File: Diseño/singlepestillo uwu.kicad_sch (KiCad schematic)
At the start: 17 parts, among them J1 MAX98357A, J2 Conn_01x03_Pin, J3 Screw_Terminal_01x03, J5 Screw_Terminal_01x02, J9 Screw_Terminal_01x03, K3 G6AU, Q6 MMBT2222A, U3 EL817, U5 L7805, U6 ESP32DevKitv1

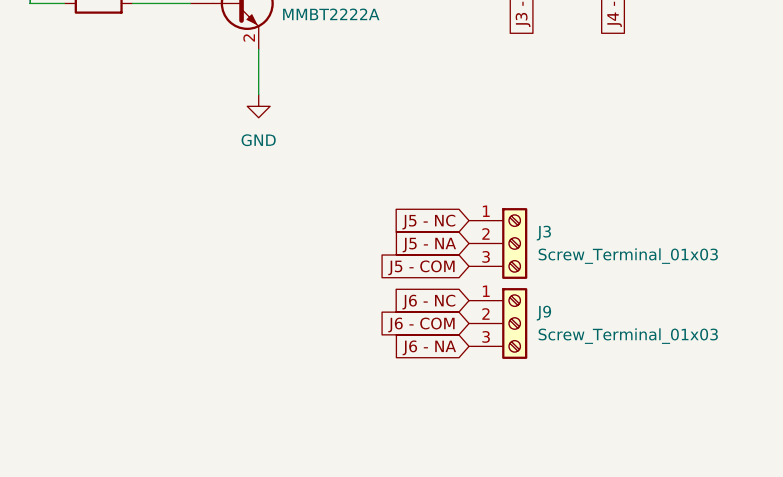
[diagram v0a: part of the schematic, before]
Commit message: avance pcb armado
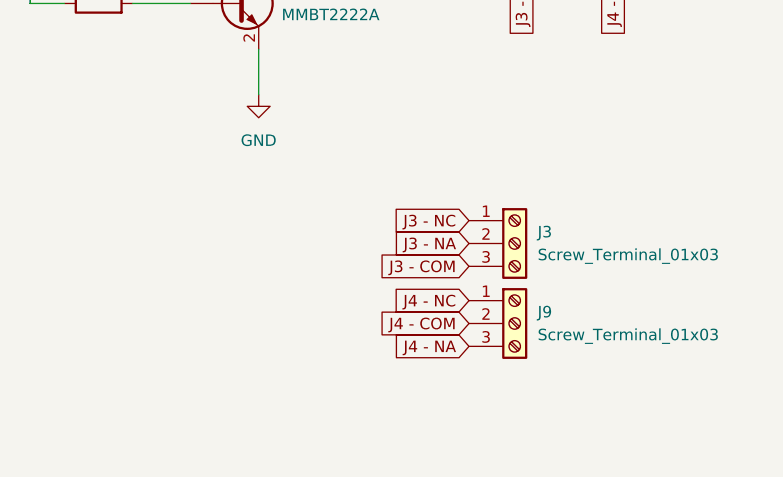
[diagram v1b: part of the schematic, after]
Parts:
- U5: footprint MacroLib:TO-220-3_Vertical -> Package_TO_SOT_THT:TO-3P-3_Vertical
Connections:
- net J5 - COM is gone; now on net J3 - COM: J3.3 (Pin_3)
- net J5 - NA is gone; now on net J3 - NA: J3.2 (Pin_2)
- net J5 - NC is gone; now on net J3 - NC: J3.1 (Pin_1)
- net J6 - COM is gone; now on net J4 - COM: J9.2 (Pin_2)
- net J6 - NA is gone; now on net J4 - NA: J9.3 (Pin_3)
- net J6 - NC is gone; now on net J4 - NC: J9.1 (Pin_1)
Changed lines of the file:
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@@
 		)
 	)
-	(global_label "J6 - NC"
+	(global_label "J4 - NC"
 		(shape input)
 		(at 255.778 90.424 180)
@@
 		)
 	)
-	(global_label "J6 - NA"
+	(global_label "J4 - NA"
 		(shape input)
 		(at 255.778 95.504 180)
@@
 		)
 	)
-	(global_label "J6 - COM"
+	(global_label "J4 - COM"
 		(shape input)
 		(at 255.778 92.964 180)
@@
 		)
 	)
-	(global_label "J5 - NA"
+	(global_label "J3 - NA"
 		(shape input)
 		(at 255.778 84.074 180)
@@
 		)
 	)
-	(global_label "J5 - COM"
+	(global_label "J3 - COM"
 		(shape input)
 		(at 255.778 86.614 180)
@@
 		)
 	)
-	(global_label "J5 - NC"
+	(global_label "J3 - NC"
 		(shape input)
 		(at 255.778 81.534 180)
@@
 			)
 		)
-		(property "Footprint" "MacroLib:TO-220-3_Vertical"
+		(property "Footprint" "Package_TO_SOT_THT:TO-3P-3_Vertical"
 			(at 72.263 34.544 0)
 			(effects
